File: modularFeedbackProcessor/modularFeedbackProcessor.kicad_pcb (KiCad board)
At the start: 4 copper layers, 191.5 x 124 mm, 204 parts, among them J1 Input, J10 Output, J2 Feedback, J4 Eurorack_Power_16pin_Unshroud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, J5 DryWet, J6 Rate, J7 EffectsRouteIn, J8 EffectsRouteOut, J9 EffectsDryWet, Q1 Q_PMOS_GDS, Q10 Q_PMOS_GDS, Q11 Q_NMOS_GDS, Q12 Q_PMOS_GDS, Q13 Q_PMOS_GDS, Q14 Q_NMOS_GDS, Q15 Q_PMOS_GDS, Q16 Q_NMOS_GDS, Q17 Q_PMOS_GDS, Q18 Q_NMOS_GDS, Q19 Q_PMOS_GDS, Q2 Q_NMOS_GDS, Q3 Q_PMOS_GDS, Q4 Q_PMOS_GDS, Q5 Q_NMOS_GDS, Q6 Q_PMOS_GDS, Q7 Q_NMOS_GDS, Q8 Q_PMOS_GDS, Q9 Q_NMOS_GDS, SW1 EffectsRouting, U1 TL074, U10 LM13700, U2 TL074, U3 LM13700, U4 V3205, U5 CD4046, U6 LF398_DIP8, U7 TL074, U8 LM13700, U9 TL074

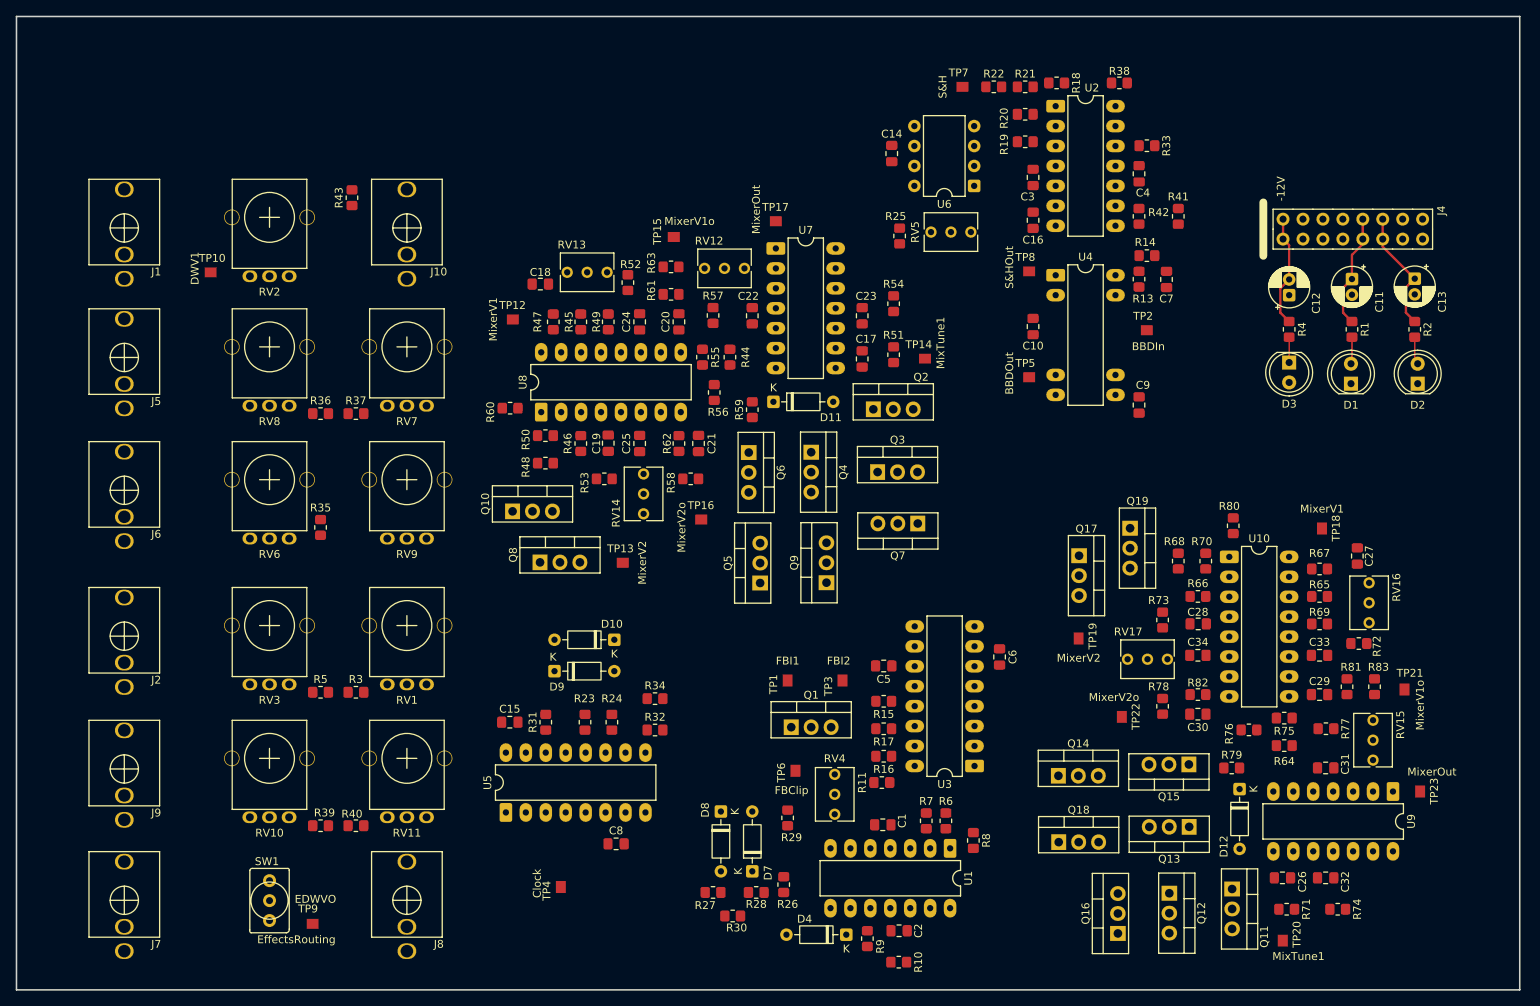
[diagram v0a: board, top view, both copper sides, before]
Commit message: mostly done with the BBD module routing
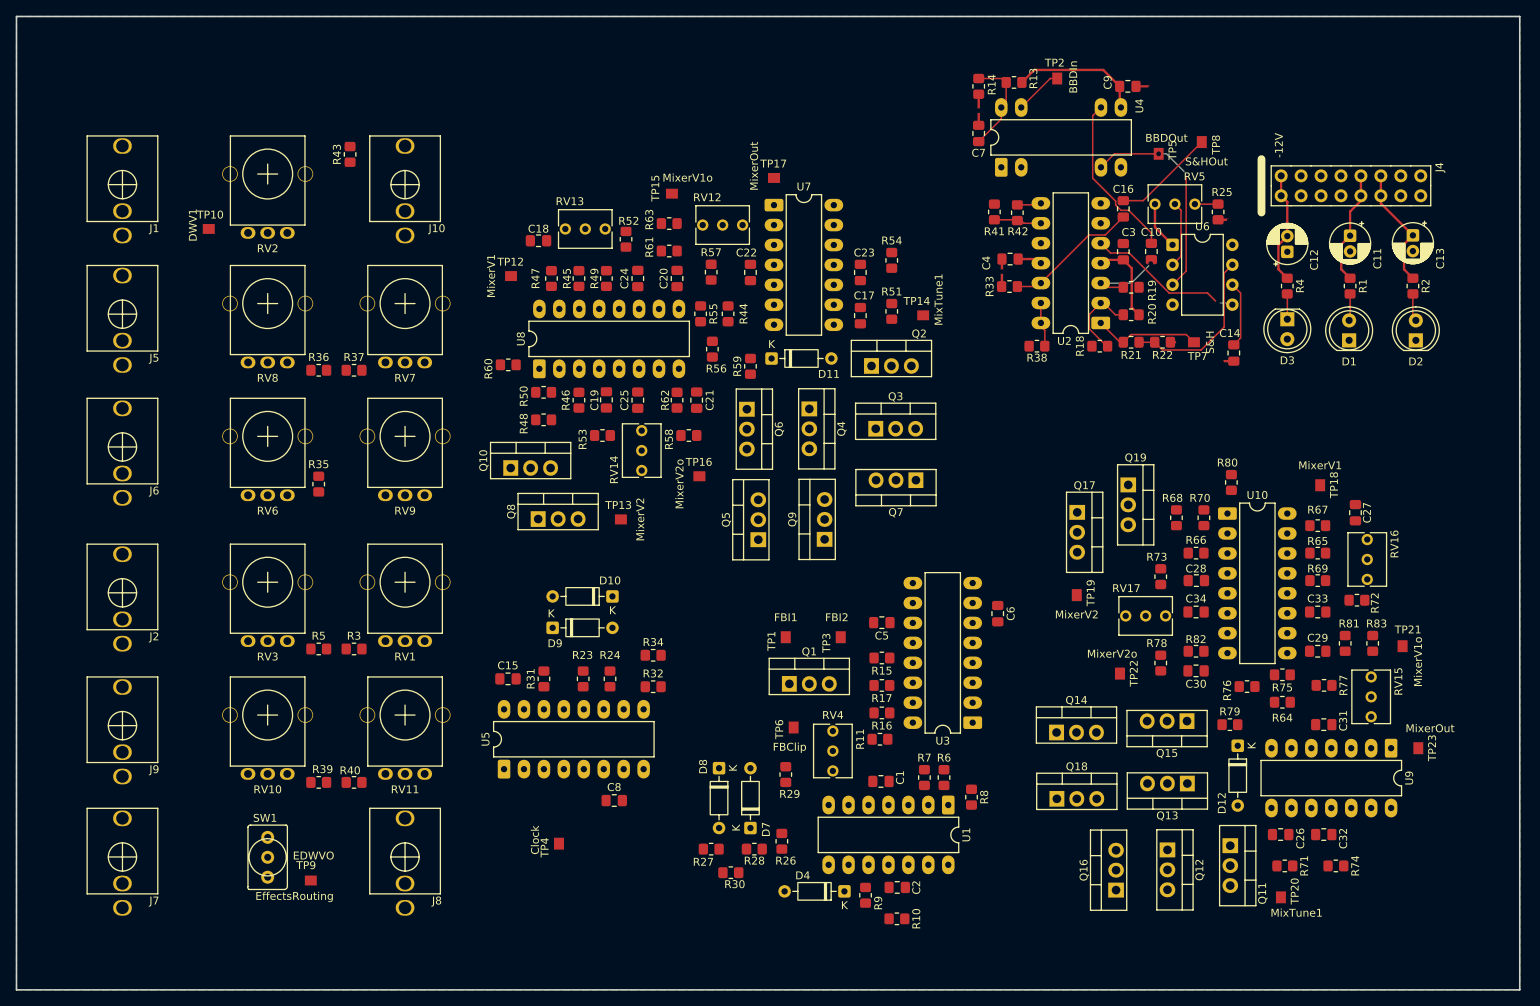
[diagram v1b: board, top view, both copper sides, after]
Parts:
- moved C14 50.4 mm to (205.1, 66.9)
- moved TP7 43.9 mm to (200.0, 65.5), turned to 180 degrees
- moved R25 40.7 mm to (203.1, 48.9)
- moved C9 40.6 mm to (191.6, 32.9), turned to 0 degrees
- moved R22 39.0 mm to (196.0, 65.5), turned to 180 degrees
- moved R21 35.2 mm to (192.0, 65.5), turned to 180 degrees
- moved R38 35.1 mm to (180.0, 66.0), turned to 180 degrees
- moved TP2 34.0 mm to (182.6, 31.9), turned to 90 degrees
- moved R18 34.0 mm to (188.0, 66.0), turned to 0 degrees
- moved RV5 33.8 mm to (200.1, 47.9), turned to -90 degrees
- moved TP5 32.9 mm to (195.5, 41.5), turned to -90 degrees
- moved R14 30.4 mm to (172.6, 32.9), turned to -90 degrees
- moved C7 30.3 mm to (172.6, 38.9), turned to 90 degrees
- moved R13 29.7 mm to (177.1, 32.4), turned to 180 degrees
- moved R20 28.9 mm to (192.0, 62.0), turned to 0 degrees
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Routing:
- net Net-(U4-OUT1): track 0.00 -> 27.5 mm, vias 0 -> 2
- net Net-(U4-CP1): track 0.00 -> 21.4 mm
- net Net-(U6-T): track 0.00 -> 20.8 mm
- net Net-(U2B-+): track 0.00 -> 20.0 mm, vias 0 -> 1
- net Net-(U2D-+): track 0.00 -> 17.2 mm
- net +12V: track 14.5 -> 31.5 mm
- net +5V: track 15.7 -> 32.4 mm
- net Net-(R21-Pad2): track 0.00 -> 13.7 mm
- net GND: track 0.00 -> 13.5 mm, vias 0 -> 6
- net Net-(U2B--): track 0.00 -> 13.1 mm
- net Net-(U4-V_{GG}): track 0.00 -> 12.7 mm
- net Net-(U2A-+): track 0.00 -> 11.1 mm, vias 0 -> 1
- net Net-(U2A--): track 0.00 -> 10.6 mm
- net Net-(U6-Adj): track 0.00 -> 8.50 mm
- net Net-(U6-C_{h}): track 0.00 -> 8.45 mm
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- added copper zone on B.Cu, net GND
- removed copper zone on In2.Cu, net GND
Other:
- copper layers 4 -> 2

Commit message: significant progress
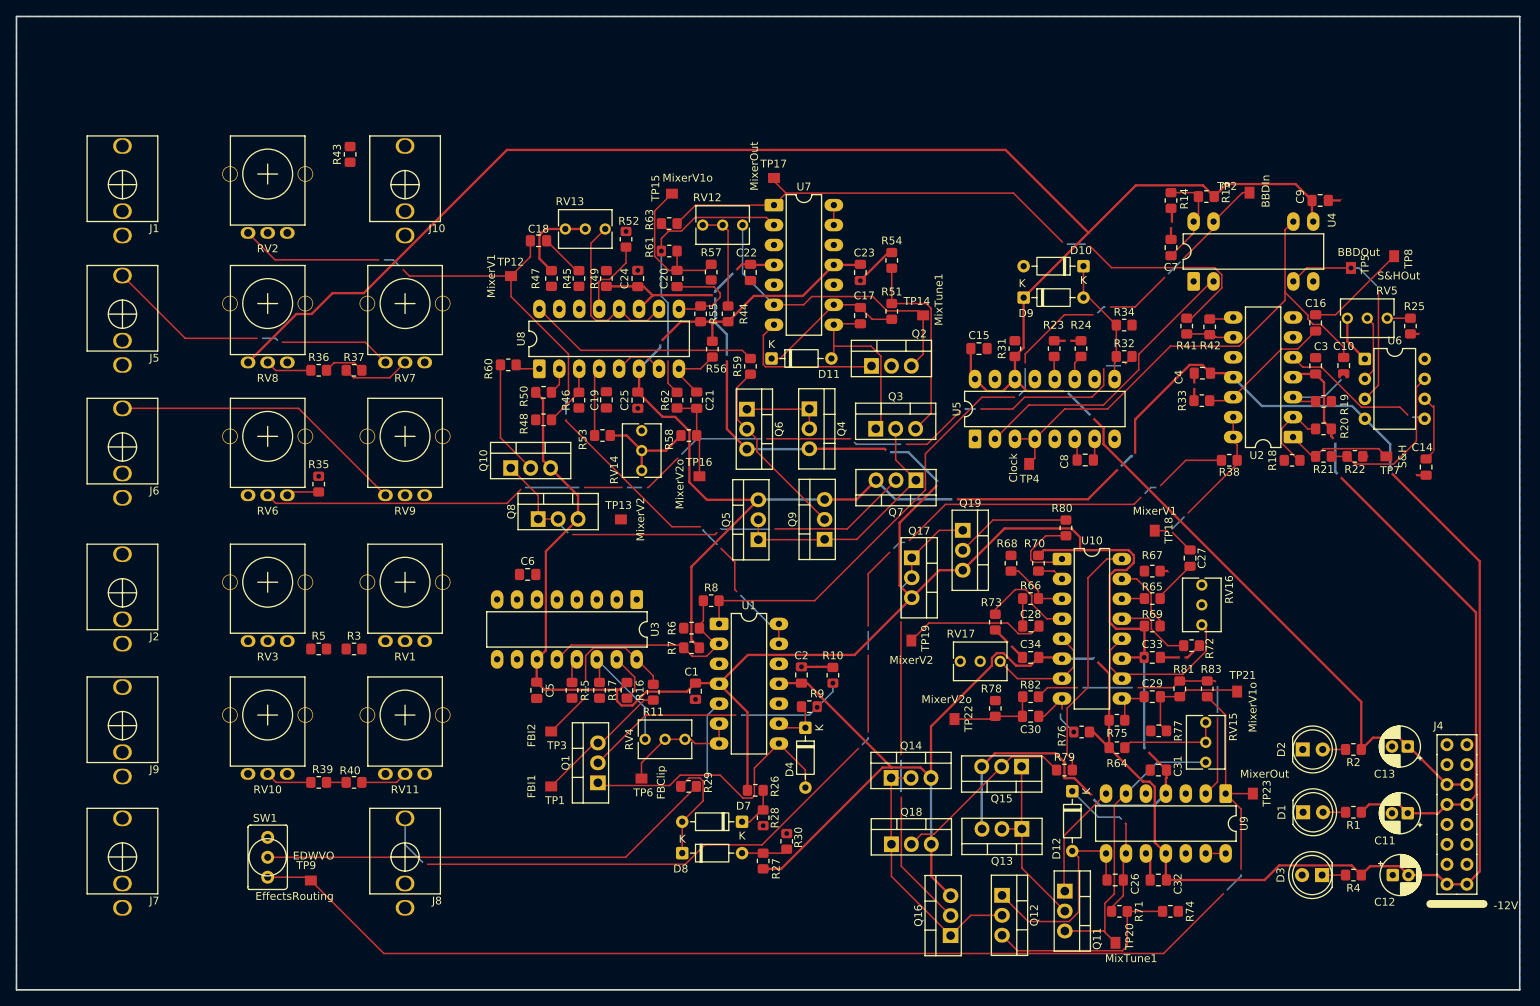
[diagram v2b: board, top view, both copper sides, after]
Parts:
- removed TP10: DWV1, PCM_4ms_TestPoint:TestPoint_Pad_06
- moved J4 81.2 mm to (233.5, 125.7), turned to 0 degrees
- moved C12 80.5 mm to (225.3, 133.4), turned to 0 degrees
- moved TP4 77.0 mm to (179.0, 81.0)
- moved R4 75.5 mm to (220.3, 133.4), turned to 180 degrees
- moved C8 74.0 mm to (186.1, 80.5)
- moved C11 73.9 mm to (227.2, 125.5), turned to 180 degrees
- moved C15 73.3 mm to (172.6, 66.3)
- moved D9 73.3 mm to (178.3, 59.8)
- moved R24 73.3 mm to (185.6, 66.3)
- moved U5 73.3 mm to (172.1, 77.8)
- moved R23 73.3 mm to (182.2, 66.3)
- moved R31 73.3 mm to (177.2, 66.3)
- moved R32 73.3 mm to (191.1, 67.3)
- moved R34 73.3 mm to (191.1, 63.3)
- moved D10 73.3 mm to (185.9, 55.8)
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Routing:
- net -12V: track 17.4 -> 417.3 mm, vias 0 -> 6
- net +12V: track 31.5 -> 410.3 mm, vias 0 -> 10
- net +5V: track 32.4 -> 276.0 mm, vias 0 -> 2
- net /Mixer2/V_{out}: track 0.00 -> 160.2 mm, vias 0 -> 2
- net Net-(J8-T): track 0.00 -> 142.0 mm, vias 0 -> 9
- net Net-(R32-Pad2): track 0.00 -> 120.4 mm, vias 0 -> 12
- net /Mixer1/V_{in1}: track 0.00 -> 105.6 mm, vias 0 -> 7
- net Net-(U4-IN): track 6.11 -> 97.9 mm, vias 0 -> 6
- net /Mixer1/V_{out}: track 0.00 -> 85.6 mm, vias 0 -> 2
- net Net-(SW1-B): track 0.00 -> 58.4 mm
- net Net-(Q10-G): track 0.00 -> 57.5 mm, vias 0 -> 3
- net Net-(Q16-D): track 0.00 -> 56.7 mm, vias 0 -> 3
- net GND: track 13.5 -> 67.4 mm, vias 6 -> 20
- net Net-(U4-CP1): track 21.4 -> 67.7 mm
- net Net-(Q2-S): track 0.00 -> 39.3 mm
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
